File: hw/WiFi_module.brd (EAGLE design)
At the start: 25 x 45 mm, 34 parts, among them J1 R2P_BUS-VERTICAL, J2 R2P_BUS-VERTICAL, X1 MOLEX_53047-04

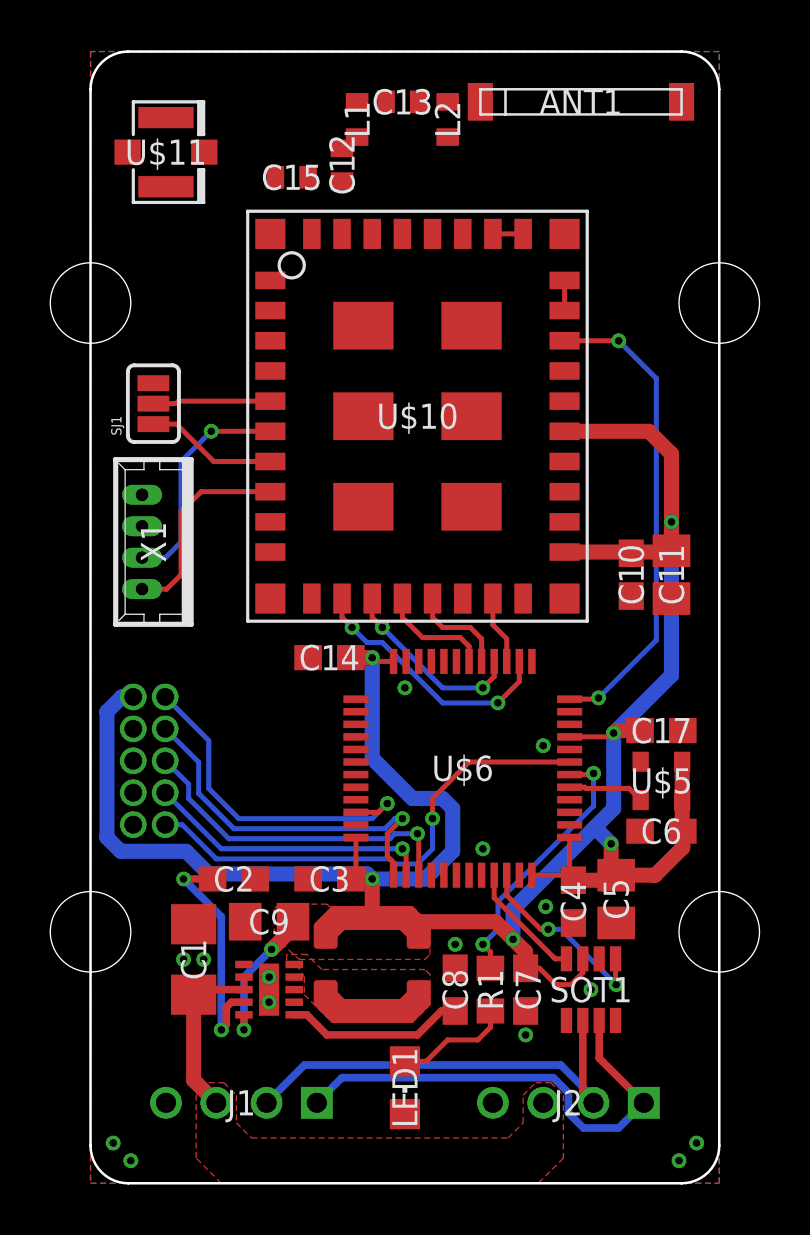
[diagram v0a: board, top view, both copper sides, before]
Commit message: Layout complete
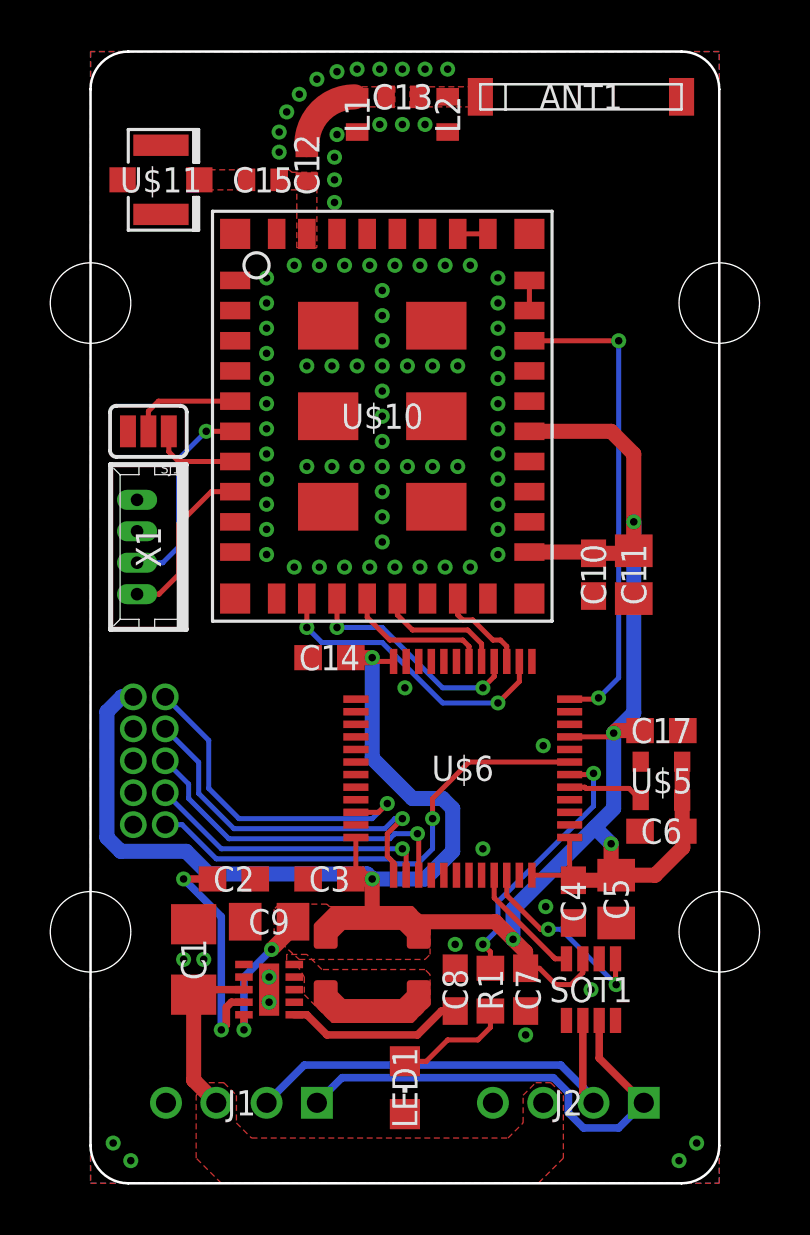
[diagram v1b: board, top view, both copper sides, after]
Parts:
- moved C10 1.50 mm to (20.0, 24.2)
- moved C11 1.50 mm to (21.6, 24.2)
- moved C12 1.40 mm to (8.60, 40.5)
- moved U$10 1.40 mm to (11.6, 30.5)
- moved C15 1.15 mm to (6.85, 39.9)
- moved SJ1 1.12 mm to (2.30, 29.9), turned to 180 degrees
- moved U$11 1.12 mm to (2.80, 39.9)
- moved X1 0.28 mm to (2.30, 25.3)
- moved ANT1 0.20 mm to (19.5, 43.2)
- moved C13 0.20 mm to (12.4, 43.2)
- moved L1 0.20 mm to (10.6, 42.5)
- moved L2 0.20 mm to (14.2, 42.5)
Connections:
- net N$21: now also C15.1
- net N$6: no longer C15.1
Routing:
- net N$6: track 0.00 -> 2.79 mm
- net N$3: track 5.27 -> 3.61 mm
- net SPI_CS: track 10.4 -> 12.0 mm
- net SPI_MISO: track 7.55 -> 9.18 mm
- net DEBUG_RX: track 8.17 -> 6.76 mm
- net SPI_IRQ: track 4.48 -> 5.88 mm
- net SPI_MOSI: track 3.95 -> 5.18 mm
- net SPI_SCK: track 2.73 -> 3.72 mm
- net DEBUG_TX: track 9.06 -> 8.11 mm
- net +3V3: track 100.9 -> 100.1 mm
- added copper zone on layer 1, net N$10
- added copper zone on layer 1, net N$21
- added copper zone on layer 1, net N$6
- added copper zone on layer 1, net N$9

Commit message: Fixed silkscreen
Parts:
- U$5: value ABRACON_ASD -> OSC; device r2p_ic:ABRACON_2.5X2 -> r2p_ic:XTAL_2.5X2
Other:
- board text added: "RF module v1.0 (2015/02)"
- board text removed: "R2P module v0.0 (YYYY/MM)"
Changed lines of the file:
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@@
 <grid distance="0.5" unitdist="mm" unit="mm" style="dots" multiple="1" display="yes" altdistance="0.1" altunitdist="mm" altunit="mm"/>
 <layers>
-<layer number="1" name="Top" color="4" fill="1" visible="yes" active="yes"/>
-<layer number="16" name="Bottom" color="1" fill="1" visible="no" active="yes"/>
+<layer number="1" name="Top" color="4" fill="1" visible="no" active="yes"/>
+<layer number="16" name="Bottom" color="1" fill="1" visible="yes" active="yes"/>
 <layer number="17" name="Pads" color="2" fill="1" visible="yes" active="yes"/>
 <layer number="18" name="Vias" color="2" fill="1" visible="yes" active="yes"/>
 <layer number="19" name="Unrouted" color="6" fill="1" visible="yes" active="yes"/>
 <layer number="20" name="Dimension" color="15" fill="1" visible="yes" active="yes"/>
-<layer number="21" name="tPlace" color="7" fill="1" visible="yes" active="yes"/>
-<layer number="22" name="bPlace" color="7" fill="1" visible="no" active="yes"/>
-<layer number="23" name="tOrigins" color="15" fill="1" visible="yes" active="yes"/>
-<layer number="24" name="bOrigins" color="15" fill="1" visible="no" active="yes"/>
+<layer number="21" name="tPlace" color="7" fill="1" visible="no" active="yes"/>
+<layer number="22" name="bPlace" color="7" fill="1" visible="yes" active="yes"/>
+<layer number="23" name="tOrigins" color="15" fill="1" visible="no" active="yes"/>
+<layer number="24" name="bOrigins" color="15" fill="1" visible="yes" active="yes"/>
 <layer number="25" name="tNames" color="7" fill="1" visible="no" active="yes"/>
 <layer number="26" name="bNames" color="7" fill="1" visible="no" active="yes"/>
@@
 <layer number="37" name="tTest" color="7" fill="1" visible="no" active="yes"/>
 <layer number="38" name="bTest" color="7" fill="1" visible="no" active="yes"/>
-<layer number="39" name="tKeepout" color="4" fill="11" visible="yes" active="yes"/>
-<layer number="40" name="bKeepout" color="1" fill="11" visible="no" active="yes"/>
-<layer number="41" name="tRestrict" color="4" fill="10" visible="yes" active="yes"/>
-<layer number="42" name="bRestrict" color="1" fill="10" visible="no" active="yes"/>
+<layer number="39" name="tKeepout" color="4" fill="11" visible="no" active="yes"/>
+<layer number="40" name="bKeepout" color="1" fill="11" visible="yes" active="yes"/>
+<layer number="41" name="tRestrict" color="4" fill="10" visible="no" active="yes"/>
+<layer number="42" name="bRestrict" color="1" fill="10" visible="yes" active="yes"/>
 <layer number="43" name="vRestrict" color="2" fill="10" visible="no" active="yes"/>
 <layer number="44" name="Drills" color="7" fill="1" visible="no" active="yes"/>
@@
 <layer number="46" name="Milling" color="3" fill="1" visible="yes" active="yes"/>
 <layer number="47" name="Measures" color="7" fill="1" visible="yes" active="yes"/>
-<layer number="48" name="Document" color="7" fill="1" visible="yes" active="yes"/>
+<layer number="48" name="Document" color="7" fill="1" visible="no" active="yes"/>
 <layer number="49" name="Reference" color="7" fill="1" visible="no" active="yes"/>
 <layer number="50" name="dxf" color="7" fill="1" visible="no" active="no"/>
-<layer number="51" name="tDocu" color="7" fill="1" visible="yes" active="yes"/>
-<layer number="52" name="bDocu" color="7" fill="1" visible="no" active="yes"/>
+<layer number="51" name="tDocu" color="7" fill="1" visible="no" active="yes"/>
+<layer number="52" name="bDocu" color="7" fill="1" visible="yes" active="yes"/>
 <layer number="53" name="tGND_GNDA" color="7" fill="1" visible="no" active="no"/>
 <layer number="54" name="bGND_GNDA" color="7" fill="1" visible="no" active="no"/>
@@
 <layer number="155" name="FabDoc3" color="7" fill="1" visible="no" active="yes"/>
 <layer number="199" name="Contour" color="7" fill="1" visible="no" active="yes"/>
-<layer number="200" name="200bmp" color="7" fill="1" visible="no" active="yes"/>
+<layer number="200" name="200bmp" color="7" fill="1" visible="yes" active="yes"/>
 <layer number="201" name="201bmp" color="7" fill="1" visible="no" active="yes"/>
 <layer number="202" name="202bmp" color="7" fill="1" visible="no" active="yes"/>
@@
 <wire x1="6.55" y1="8" x2="6.55" y2="8.8" width="0.2" layer="41"/>
 <wire x1="6.55" y1="8.8" x2="7.45" y2="8.8" width="0.2" layer="41"/>
-<text x="4" y="6" size="1.5" layer="200" rot="MR90">R2P module
-v0.0 (YYYY/MM)</text>
+<text x="4" y="6" size="1.5" layer="200" rot="MR90">RF module
+v1.0 (2015/02)</text>
 <polygon width="0.2" layer="41">
 <vertex x="25" y="45"/>
@@
 </element>
 <element name="U$1" library="r2p_pcb" package="25X45" value="PCB_25X45" x="0" y="0" smashed="yes"/>
-<element name="U$5" library="r2p_ic" package="ABRACON_2.5X2" value="ABRACON_ASD" x="22.7" y="16" smashed="yes" rot="R180">
+<element name="U$5" library="r2p_ic" package="XTAL_2.5X2" value="OSC" x="22.7" y="16" smashed="yes" rot="R180">
 <attribute name="NAME" x="22.7" y="16" size="1" layer="25" font="vector" rot="R180" align="center"/>
 <attribute name="VALUE" x="24.95" y="18.75" size="1.27" layer="27" rot="R180"/>
